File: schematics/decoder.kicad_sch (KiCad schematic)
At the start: 5 parts, among them U10 ATF22V10C-7, U11 74HC373, U29 74HC245, U9 ATF22V10C-7

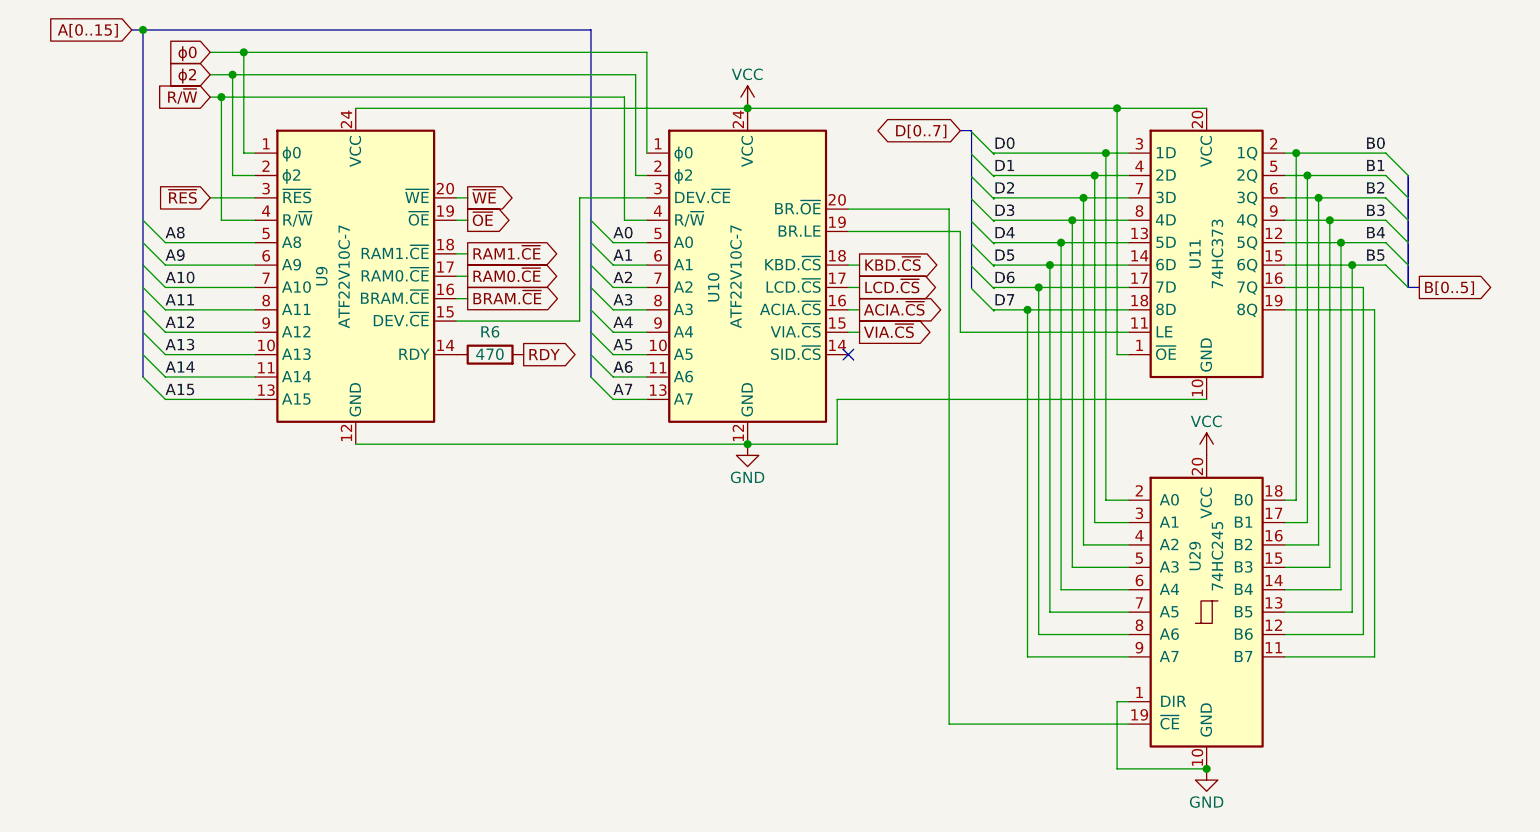
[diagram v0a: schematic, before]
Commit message: clock improvements
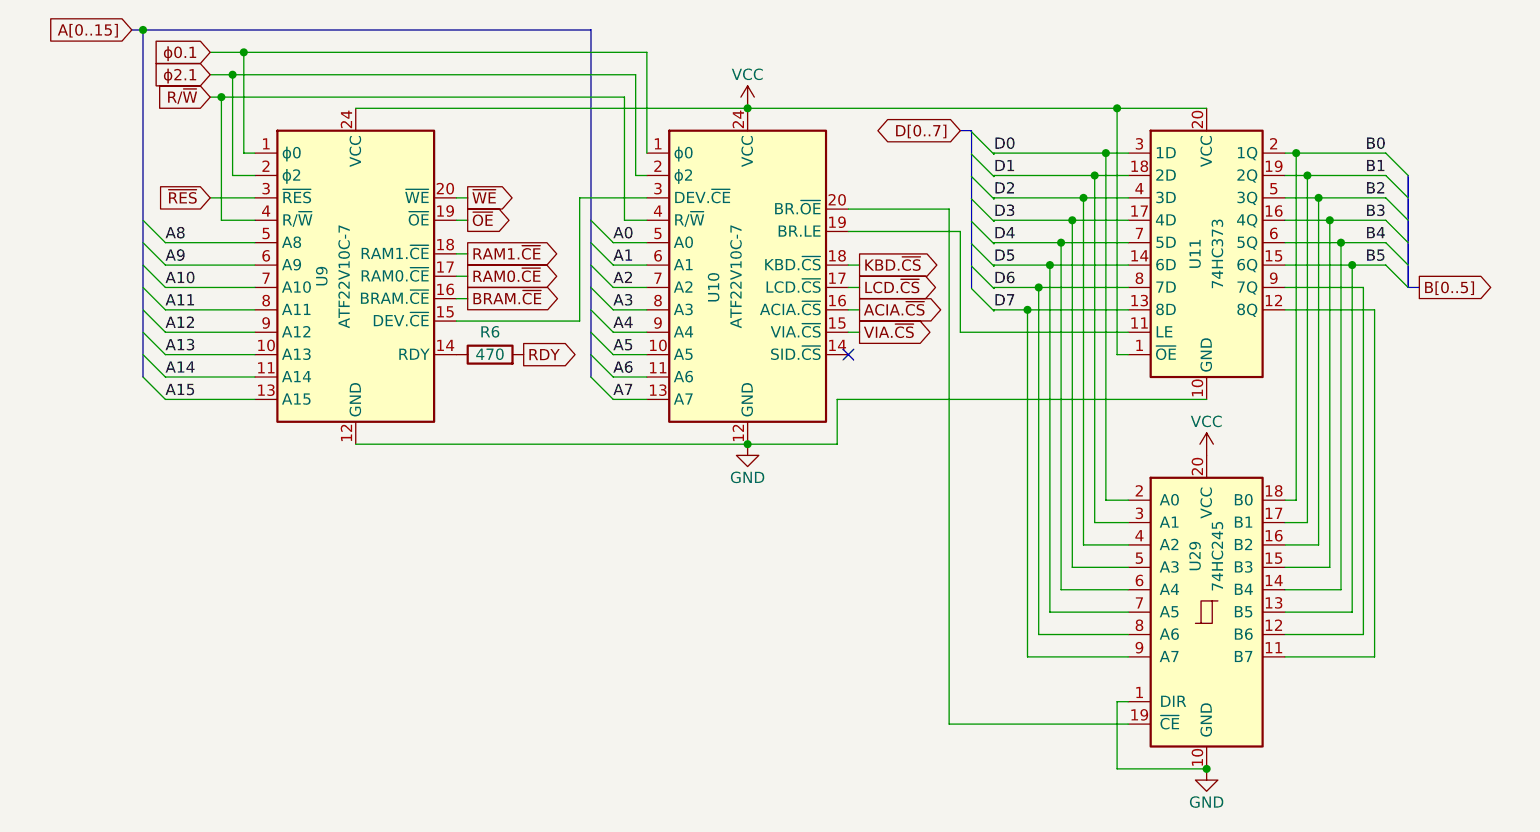
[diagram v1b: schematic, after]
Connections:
- net B1: now also U11.19 (2Q); no longer U11.5 (2Q)
- net B2: now also U11.5 (3Q); no longer U11.6 (3Q)
- net B3: now also U11.16 (4Q); no longer U11.9 (4Q)
- net B4: now also U11.6 (5Q); no longer U11.12 (5Q)
- net D1: now also U11.18 (2D); no longer U11.4 (2D)
- net D2: now also U11.4 (3D); no longer U11.7 (3D)
- net D3: now also U11.17 (4D); no longer U11.8 (4D)
- net D4: now also U11.7 (5D); no longer U11.13 (5D)
- net D6: now also U11.8 (7D); no longer U11.17 (7D)
- net D7: now also U11.13 (8D); no longer U11.18 (8D)
- net at U29.12 (B6): now also U11.9 (7Q); no longer U11.16 (7Q)
- net at U29.11 (B7): now also U11.12 (8Q); no longer U11.19 (8Q)
- net ϕ0 renamed ϕ0.1
- net ϕ2 renamed ϕ2.1
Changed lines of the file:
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@@
 		)
 	)
-	(global_label "ϕ2"
+	(global_label "ϕ2.1"
 		(shape input)
 		(at 74.93 64.77 180)
@@
 		)
 		(property "Intersheetrefs" "${INTERSHEET_REFS}"
-			(at 69.4048 64.77 0)
+			(at 67.5905 64.77 0)
 			(hide yes)
 			(show_name no)
@@
 		)
 	)
-	(global_label "ϕ0"
+	(global_label "ϕ0.1"
 		(shape input)
 		(at 74.93 62.23 180)
@@
 		)
 		(property "Intersheetrefs" "${INTERSHEET_REFS}"
-			(at 69.4048 62.23 0)
+			(at 67.5905 62.23 0)
 			(hide yes)
 			(show_name no)
